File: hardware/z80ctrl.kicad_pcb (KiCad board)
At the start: 2 copper layers, 99.8 x 49.9 mm, 31 parts, among them J1 BUS, J2 BUSEXT, J3 ISP, J4 IOADDR, J5 SERIAL1, J6 SERIAL2, J7 Pololu SD, J8 Adafruit SD, J9 CLK/WAIT, SW1 RESET, SW2 HALT, U1 74HCT139, U2 ATMEGA1284P-PU, U3 74HCT02, U4 MCP23S17, Y1 20MHz

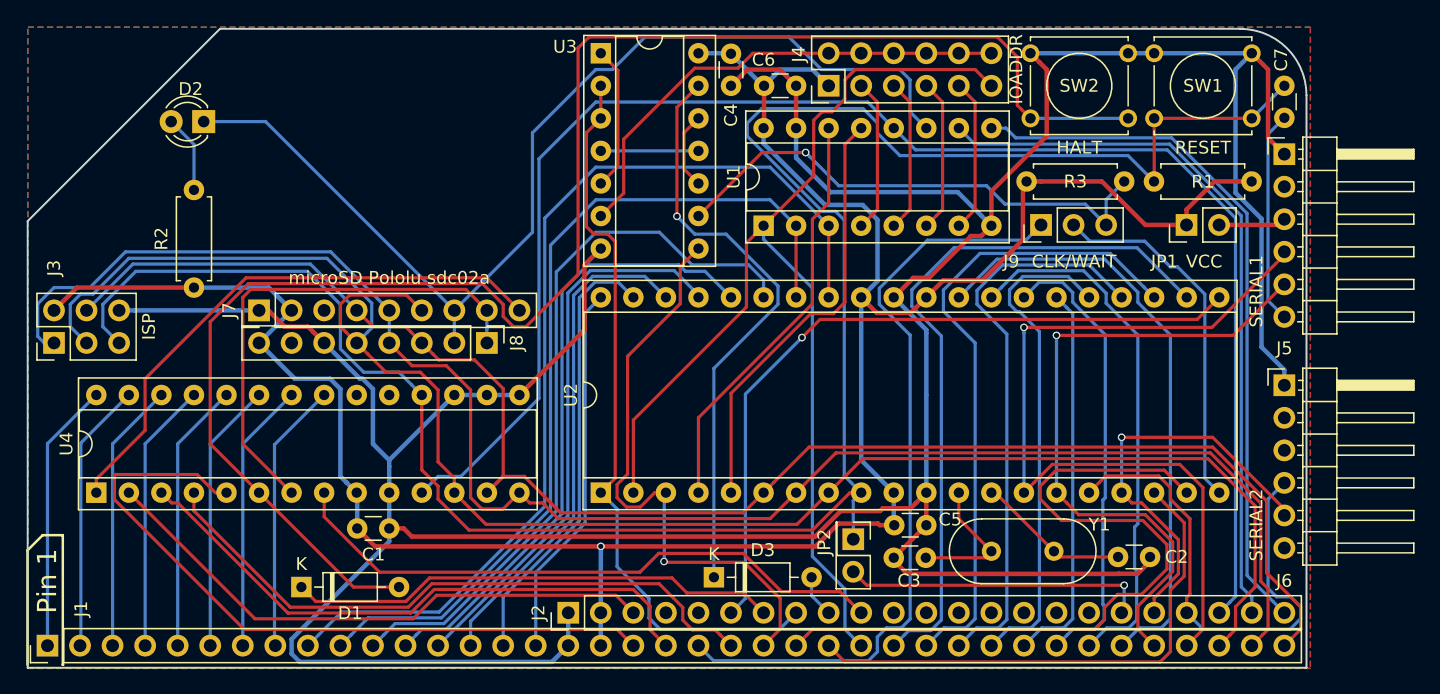
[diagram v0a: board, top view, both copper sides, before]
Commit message: Updated REV5 PCB/schematics
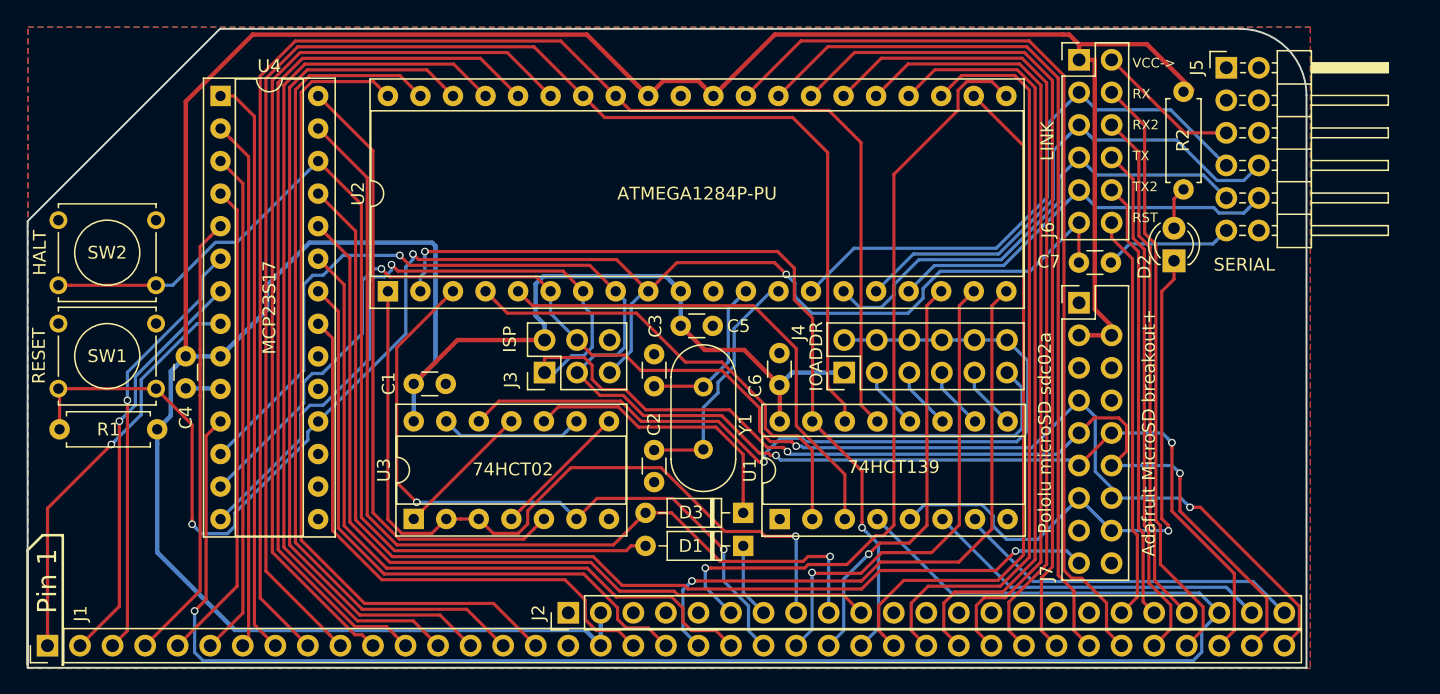
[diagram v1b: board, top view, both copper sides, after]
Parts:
- removed J8: Adafruit SD, Connector_PinHeader_2.54mm:PinHeader_1x08_P2.54mm_Vertical
- removed J9: CLK/WAIT, Connector_PinHeader_2.54mm:PinHeader_1x03_P2.54mm_Vertical
- removed JP1: VCC, Connector_PinHeader_2.54mm:PinHeader_1x02_P2.54mm_Vertical
- removed JP2: Jumper, Connector_PinHeader_2.54mm:PinHeader_2x01_P2.54mm_Vertical
- removed R3: 10K, Resistor_THT:R_Axial_DIN0207_L6.3mm_D2.5mm_P7.62mm_Horizontal
- J5: value SERIAL1 -> SERIAL; footprint Connector_PinHeader_2.54mm:PinHeader_1x06_P2.54mm_Horizontal -> Connector_PinHeader_2.54mm:PinHeader_2x06_P2.54mm_Horizontal
- J6: value SERIAL2 -> LINK; footprint Connector_PinHeader_2.54mm:PinHeader_1x06_P2.54mm_Horizontal -> Connector_PinHeader_2.54mm:PinHeader_2x06_P2.54mm_Vertical
- J7: value Pololu SD -> SD; footprint custom:microSD_Breakout_VR_LS -> Connector_PinHeader_2.54mm:PinHeader_2x09_P2.54mm_Vertical
- moved SW1 88.1 mm to (156.6, 126.5)
- moved R1 87.6 mm to (164.3, 134.8)
- moved R2 77.2 mm to (244.4, 116.0), turned to 90 degrees
- moved SW2 77.0 mm to (156.6, 118.4)
- moved D2 76.5 mm to (243.6, 121.6), turned to 90 degrees
- moved J7 64.0 mm to (236.2, 124.9), turned to 0 degrees
- moved C4 48.7 mm to (166.5, 129.1)
- moved U3 39.2 mm to (184.3, 141.8), turned to 90 degrees
- moved J3 38.4 mm to (194.5, 130.3)
- moved C2 37.1 mm to (203.0, 136.4), turned to 270 degrees
- moved D1 34.6 mm to (210.0, 143.9), turned to 180 degrees
- moved U4 32.4 mm to (169.2, 108.7), turned to 0 degrees
- moved J6 30.0 mm to (236.2, 105.9)
- moved Y1 28.5 mm to (206.9, 136.3), turned to 90 degrees
- moved C3 25.1 mm to (203.0, 131.4), turned to 90 degrees
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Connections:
- J1 pad 35: /TX -> /TXb
- J1 pad 36: /RX -> /RXb
- J2 pad 18: Net-(J2-Pad18) -> /~AVRRSTb~
- J2 pad 19: /TX2 -> /TX2b
- J2 pad 20: /RX2 -> /RX2b
- J2 pad 3: /~RFSH~ -> (no net)
- J5 pad 2: (no net) -> GND
- J5 pad 3: Net-(J5-Pad3) -> (no net)
- J5 pad 4: /RX -> (no net)
- J5 pad 5: /TX -> /VCCs
- J5 pad 6: Net-(C7-Pad1) -> (no net)
- J6 pad 1: GND -> VCC
- J6 pad 2: (no net) -> /VCCs
- J6 pad 3: (no net) -> /RX
- J6 pad 4: /RX2 -> /RXb
- J6 pad 5: /TX2 -> /RX2
- J6 pad 6: (no net) -> /RX2b
- J7 pad 3: (no net) -> VCC
- J7 pad 4: /MOSI -> VCC
- J7 pad 5: /MISO -> (no net)
- J7 pad 6: /SCK -> (no net)
- J7 pad 7: /~SDCS~ -> /MOSI
- J7 pad 8: /~SDCD~ -> GND
- J7 pad 9: /SDEN -> /MISO
- U1 pad 1: /~IORQ~ -> GND
- U1 pad 10: /~AUXCS1~ -> Net-(J4-Pad7)
- U1 pad 11: /~SDCS~ -> Net-(J4-Pad5)
- U1 pad 12: /~IOXCS~ -> Net-(J4-Pad3)
- U1 pad 13: /SPIA1 -> /A7
- U1 pad 14: /SPIA0 -> /A6
- U1 pad 15: GND -> /~IORQ~
- U1 pad 2: /A6 -> /SPIA0
- U1 pad 3: /A7 -> /SPIA1
- U1 pad 4: Net-(J4-Pad3) -> /~IOXCS~
- U1 pad 5: Net-(J4-Pad5) -> /~SDCS~
- U1 pad 6: Net-(J4-Pad7) -> /~AUXCS1~
- U1 pad 7: Net-(J4-Pad9) -> /~AUXCS2~
- U1 pad 9: /~AUXCS2~ -> Net-(J4-Pad9)
- U2 pad 20: Net-(J9-Pad2) -> /CLK
- U3 pad 10: Net-(U3-Pad10) -> Net-(D3-Pad1)
- U3 pad 11: Net-(U3-Pad11) -> Net-(U3-Pad1)
- U3 pad 12: Net-(U3-Pad10) -> Net-(J4-Pad10)
- U3 pad 13: Net-(D3-Pad1) -> Net-(U3-Pad13)
- U3 pad 4: Net-(U3-Pad11) -> Net-(U3-Pad4)
- U3 pad 5: Net-(U3-Pad1) -> /~MWAIT~
- U3 pad 6: Net-(J4-Pad10) -> /~MREQ~
- U3 pad 8: /~MREQ~ -> Net-(U3-Pad4)
- U3 pad 9: /~MWAIT~ -> Net-(U3-Pad13)
- U4 pad 1: /SDEN -> /A8
- U4 pad 2: /~RFSH~ -> /A9
- U4 pad 21: /A8 -> /~M1~
- U4 pad 22: /A9 -> /~RST~
- U4 pad 23: /A10 -> /~INT~
- U4 pad 24: /A11 -> /~NMI~
- U4 pad 25: /A12 -> /SDEN
- U4 pad 26: /A13 -> Net-(D1-Pad2)
- U4 pad 27: /A14 -> /~WAIT~
- U4 pad 28: /A15 -> /~MWAIT~
- U4 pad 3: /~RST~ -> /A10
- U4 pad 4: /~INT~ -> /A11
- U4 pad 5: /~M1~ -> /A12
- U4 pad 6: Net-(D1-Pad2) -> /A13
- U4 pad 7: /~SDCD~ -> /A14
- U4 pad 8: /~NMI~ -> /A15
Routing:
- net GND: track 296.2 -> 2.73 mm
- net VCC: track 188.9 -> 278.5 mm, vias 1 -> 0
- net /~WAIT~: track 3.32 -> 76.0 mm, vias 0 -> 1
- net Net-(D1-Pad2): track 128.2 -> 76.9 mm
- net /A6: track 68.5 -> 116.5 mm
- net /RXb: track 0.00 -> 46.7 mm
- net /~AVRRST~: track 169.3 -> 124.1 mm, vias 0 -> 3
- net /~RFSH~: track 44.8 -> 0.00 mm
- net /A7: track 76.8 -> 119.6 mm
- net /SDEN: track 44.5 -> 87.0 mm, vias 0 -> 1
- net /TXb: track 0.00 -> 40.5 mm
- net /RX2b: track 0.00 -> 40.5 mm
- net /~SDCD~: track 39.3 -> 0.00 mm
- net /~SDCS~: track 82.8 -> 46.3 mm, vias 0 -> 1
- net /A0: track 29.3 -> 64.2 mm
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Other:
- board text added: "Adafruit MicroSD breakout+"
- board text added: "Pololu microSD sdc02a"
- board text added: "VCC-> RX RX2 TX TX2 RST"
- board text added: "z80ctrl REV5 (C)2020 J.B. Langston https://github.com/jblang/z80ctrl"
- board text removed: "J4: IO addresses - None (left) - 00-3F - 40-7F - 80-BF - C0-FF - 00-FF (right) JP1: VCC from SERIAL1 JP2: VCC from SERIAL2"
- board text removed: "microSD Pololu sdc02a"
- board text removed: "z80ctrl REV4 (C)2018 J.B. Langston https://github.com/jblang/z80ctrl"
